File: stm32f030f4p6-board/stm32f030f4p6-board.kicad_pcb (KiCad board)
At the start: 4 copper layers, 29 x 31.2 mm, 19 parts, among them J1 SWD_Power, J2 Boot0_selector, J3 Conn_01x07_Pin, J5 Conn_01x07_Pin, SW1 MCU_reset, U1 STM32F030F4Px, Y1 8Mhz

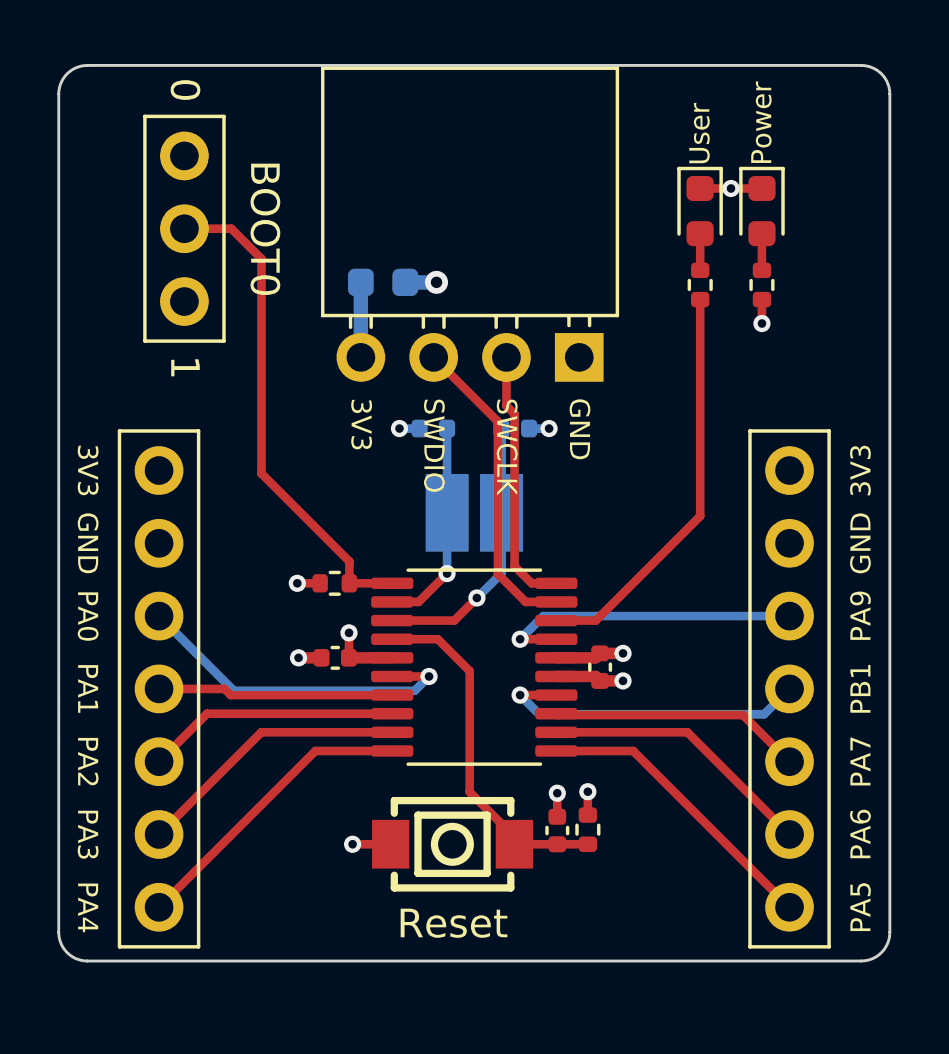
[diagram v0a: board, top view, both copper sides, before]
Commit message: ---
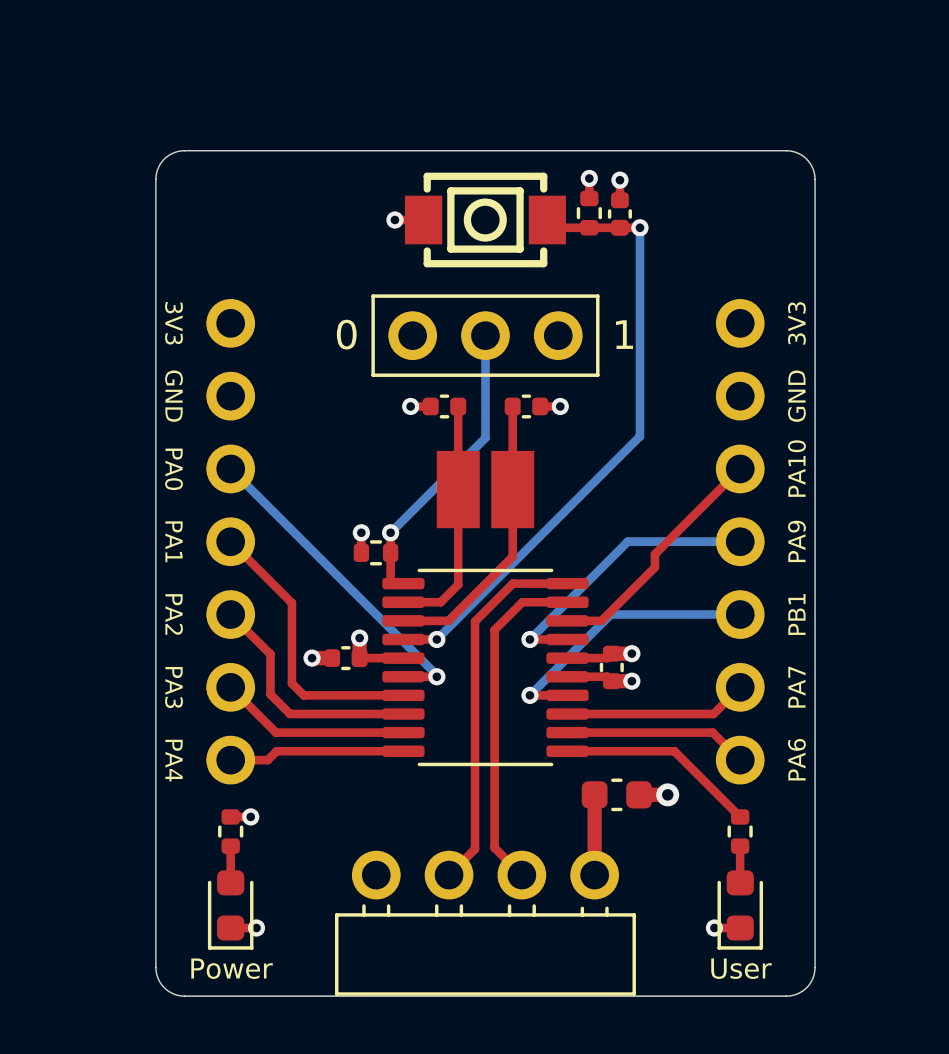
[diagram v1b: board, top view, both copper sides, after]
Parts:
- C1, C2, C5, Y1: moved to F.Cu
- J3, J5: moved to B.Cu
- moved D1 30.5 mm to (88.0, 77.3), turned to 90 degrees
- moved R4 26.6 mm to (88.0, 74.7), turned to -90 degrees
- moved D2 24.3 mm to (105.8, 77.3), turned to 90 degrees
- moved SW1 21.8 mm to (96.9, 53.4)
- moved C6 21.6 mm to (101.6, 53.2)
- moved R3 21.5 mm to (100.5, 53.2)
- moved C5 19.7 mm to (101.5, 73.5)
- moved R5 19.1 mm to (105.8, 74.7), turned to -90 degrees
- moved J1 18.1 mm to (100.7, 76.3)
- moved J2 13.1 mm to (99.4, 57.4), turned to -90 degrees
- moved J5 5.71 mm to (88.0, 57.0), turned to 180 degrees
- moved J3 5.42 mm to (105.8, 57.0), turned to 180 degrees
- moved R1 1.79 mm to (93.1, 65.0)
- moved Y1 0.90 mm to (96.9, 62.8)
- moved C1 0.86 mm to (95.5, 59.9)
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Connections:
- J1 pad 1: GND -> +3.3V
- J1 pad 2: /SWCLK -> /SWDIO
- J1 pad 3: /SWDIO -> /SWCLK
- J1 pad 4: +3.3V -> GND
- J3 pad 3: /PA9 -> /PA10
- J3 pad 4: /PB1 -> /PA9
- J3 pad 5: /PA7 -> /PB1
- J3 pad 6: /PA6 -> /PA7
- J3 pad 7: /PA5 -> /PA6
- R5 pad 1: /PA10 -> /PA5
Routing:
- net /nrst: track 12.4 -> 21.8 mm, vias 0 -> 2
- net /boot0: track 17.2 -> 10.5 mm, vias 0 -> 1
- net /PA10: track 14.1 -> 8.49 mm
- net /PA4: track 10.4 -> 6.16 mm
- net /SWCLK: track 9.11 -> 13.0 mm
- net /PA5: track 10.4 -> 6.97 mm
- net /PA6: track 9.61 -> 6.42 mm
- net /PA3: track 9.61 -> 6.68 mm
- net /PA7: track 8.83 -> 6.41 mm
- net /PA1: track 8.23 -> 9.89 mm
- net /PB1: track 11.3 -> 9.82 mm
- net GND: track 10.8 -> 9.61 mm, vias 9 -> 10
- net Net-(U1-PF0): track 7.38 -> 8.38 mm, vias 1 -> 0
- net /SWDIO: track 10.9 -> 11.9 mm
- net /PA9: track 11.0 -> 10.1 mm
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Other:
- board size 29 x 31.2 mm -> 23 x 29.5 mm
- board text added: "CLK"
- board text added: "DIO"
- board text added: "PA10"
- board text removed: "BOOT0"
- board text removed: "PA5"
- board text removed: "Reset"
- board text removed: "SWCLK"
- board text removed: "SWDIO"
